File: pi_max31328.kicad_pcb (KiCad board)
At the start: 2 copper layers, 21.5 x 14 mm, 9 parts, among them J1 PINHD_1x5_Female, U1 MAX31328NELB+

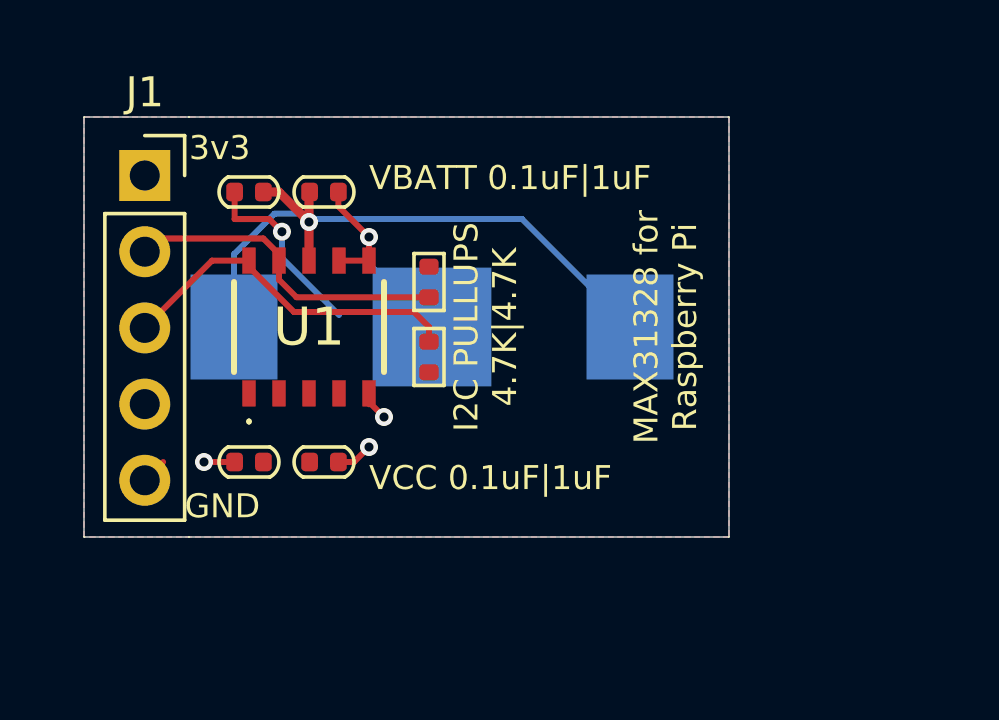
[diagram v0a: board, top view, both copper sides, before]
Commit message: v0.2
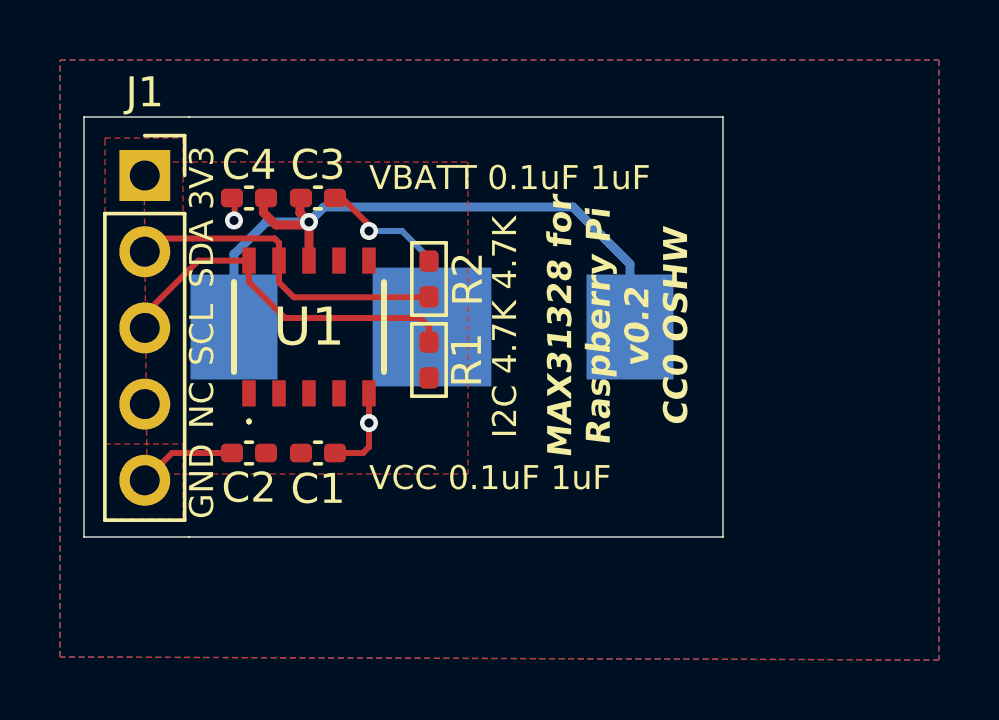
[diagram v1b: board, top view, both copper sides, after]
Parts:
- C1, C2, C3, C4: footprint PCM_Capacitor_SMD_AKL:C_0402_1005Metric -> Capacitor_SMD:C_0402_1005Metric_Pad0.74x0.62mm_HandSolder
- R1, R2: footprint PCM_Resistor_SMD_AKL:R_0402_1005Metric -> PCM_Resistor_SMD_AKL:R_0402_1005Metric_Pad0.72x0.64mm_HandSolder
- moved C1 0.36 mm to (23.8, 31.2)
- moved C2 0.30 mm to (21.5, 31.2)
- moved C3 0.28 mm to (23.8, 22.7)
- moved C4 0.20 mm to (21.5, 22.7)
- moved R1 0.10 mm to (27.5, 28.1)
- moved R2 0.10 mm to (27.5, 25.4)
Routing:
- net /GND: track 18.0 -> 14.0 mm, vias 5 -> 3
- net /VBAT: track 22.0 -> 23.6 mm
- added copper zone on F.Cu, net /GND
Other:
- board size 21.5 x 14 mm -> 21.3 x 14 mm
- board text added: "3V3"
- board text added: "I2C 4.7K 4.7K"
- board text added: "MAX31328 for Raspberry Pi v0.2 CC0 OSHW"
- board text added: "NC"
- board text added: "SCL"
- board text added: "SDA"
- board text added: "VBATT 0.1uF 1uF"
- board text added: "VCC 0.1uF 1uF"
- board text removed: "3v3"
- board text removed: "I2C PULLUPS 4.7K|4.7K"
- board text removed: "MAX31328 for Raspberry Pi"
- board text removed: "VBATT 0.1uF|1uF"
- board text removed: "VCC 0.1uF|1uF"
